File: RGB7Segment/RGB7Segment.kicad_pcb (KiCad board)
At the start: 2 copper layers, 34 x 31.5 mm, 14 parts, among them J1 Conn_01x04_Female, J2 Conn_01x04_Female

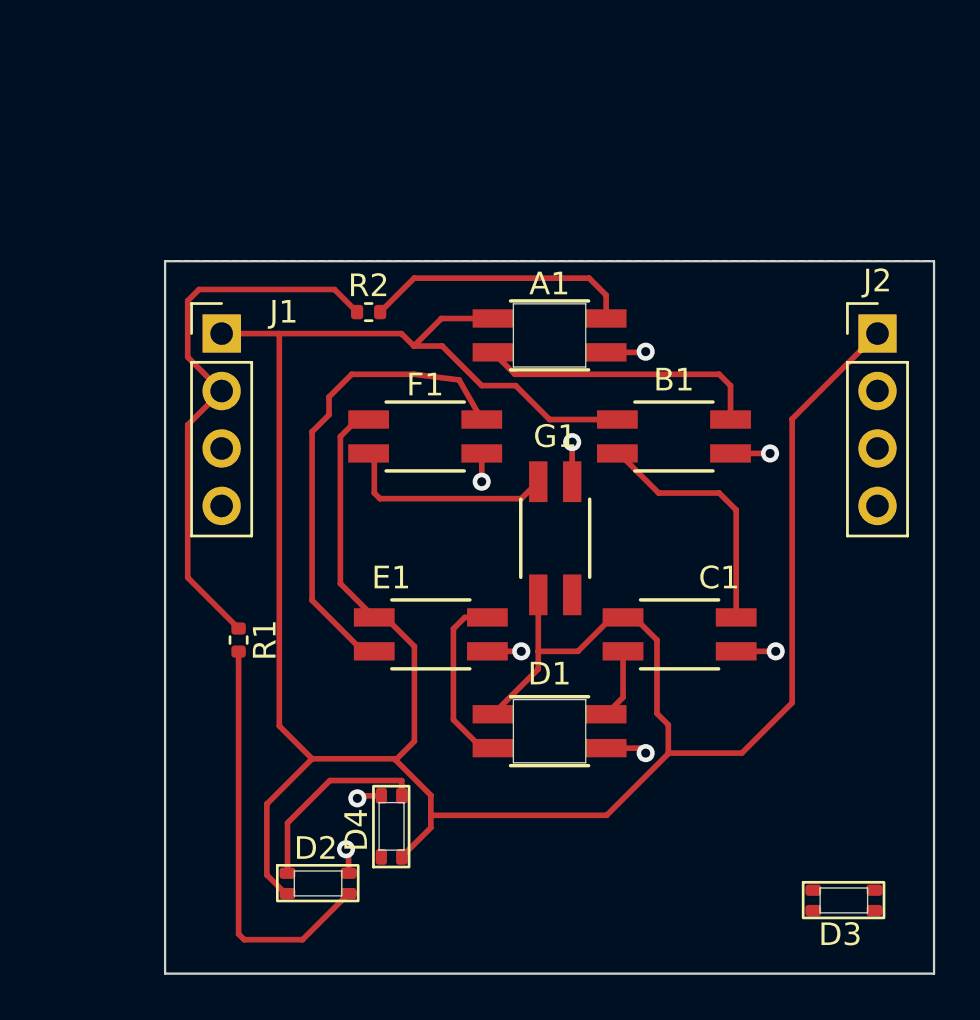
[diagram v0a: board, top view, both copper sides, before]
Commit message: Slotted/Cut Design Uploaded. Waiting on COnfirmation of Operation
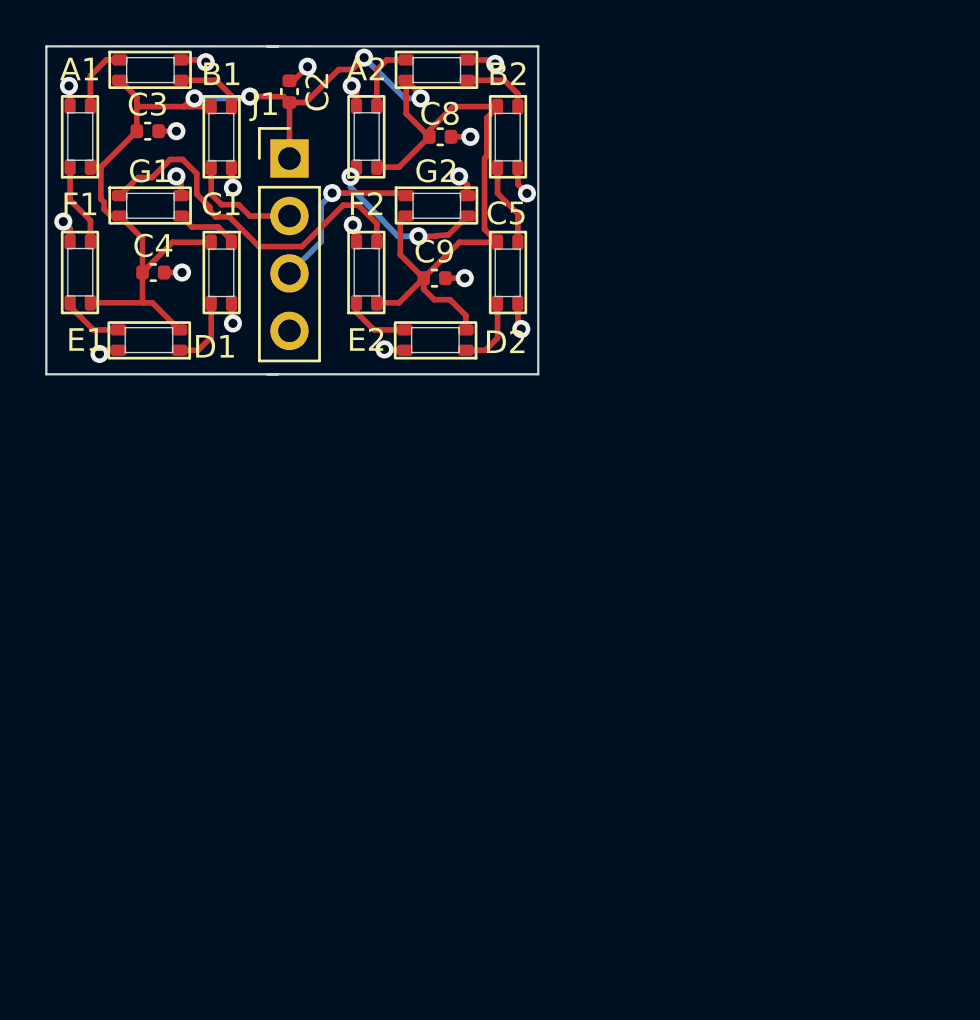
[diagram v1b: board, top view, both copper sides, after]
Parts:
- removed D3, D4: SK6812-E, Library:12-23C
- removed J2: Conn_01x04_Female, Connector_PinHeader_2.54mm:PinHeader_1x04_P2.54mm_Vertical
- removed R1, R2: 0, Resistor_SMD:R_0402_1005Metric
- added A2: SK6812-E, Library:12-23C, F.Cu at (192.7, 76.5)
- added B2: SK6812-E, Library:12-23C, F.Cu at (196.7, 77.7)
- added C2: 0.470u, Capacitor_SMD:C_0402_1005Metric, F.Cu at (187.5, 77.0)
- added C3: 0.1u, Capacitor_SMD:C_0402_1005Metric, F.Cu at (181.2, 78.8)
- added C4: 0.1u, Capacitor_SMD:C_0402_1005Metric, F.Cu at (181.5, 85.0)
- added C5: SK6812-E, Library:12-23C, F.Cu at (196.7, 83.7)
- added C8: 0.1u, Capacitor_SMD:C_0402_1005Metric, F.Cu at (194.2, 79.0)
- added C9: 0.1u, Capacitor_SMD:C_0402_1005Metric, F.Cu at (193.9, 85.2)
- added E2: SK6812-E, Library:12-23C, F.Cu at (191.4, 86.3)
- added F2: SK6812-E, Library:12-23C, F.Cu at (191.4, 80.3)
- added G2: SK6812-E, Library:12-23C, F.Cu at (192.7, 82.5)
- A1, D1: footprint Library:4960_ADA -> Library:12-23C
- B1: footprint Library:4960_Test2 -> Library:12-23C
- C1, G1: footprint Library:4960_Test4 -> Library:12-23C
- E1: footprint Library:4960_Test3 -> Library:12-23C
- F1: footprint Library:4960_Test1 -> Library:12-23C
- moved C1 27.0 mm to (184.0, 83.7), turned to -90 degrees
- moved D2 26.1 mm to (195.3, 87.5), turned to 180 degrees
- moved B1 25.1 mm to (184.0, 77.7), turned to -90 degrees
- moved D1 24.1 mm to (182.6, 87.5), turned to 180 degrees
- moved G1 24.0 mm to (180.0, 82.5), turned to 0 degrees
- moved A1 22.1 mm to (180.0, 76.5)
- moved E1 21.0 mm to (178.7, 86.3), turned to 90 degrees
- moved F1 19.0 mm to (178.7, 80.3), turned to 90 degrees
- moved J1 8.30 mm to (187.5, 80.0)
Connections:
- net +3V3 renamed VCC
- A1 pad 2: Net-(A1-Pad2) -> /F1
- A1 pad 4: Net-(R2-Pad2) -> /A1
- B1 pad 2: Net-(B1-Pad2) -> /A1
- B1 pad 4: Net-(A1-Pad2) -> /DIN
- C1 pad 2: /D1 -> /G1
- C1 pad 4: Net-(B1-Pad2) -> /C1
- D1 pad 2: Net-(D1-Pad2) -> /C1
- D2 pad 2: Net-(D2-Pad2) -> /C2
- D2 pad 4: Net-(D2-Pad4) -> /D2
- E1 pad 2: Net-(E1-Pad2) -> /D1
- E1 pad 4: Net-(D1-Pad2) -> /E1
- F1 pad 2: Net-(F1-Pad2) -> /E1
- F1 pad 4: Net-(E1-Pad2) -> /F1
- G1 pad 2: /D2 -> /E2
- G1 pad 4: Net-(F1-Pad2) -> /G1
- J1 pad 3: unconnected-(J1-Pad3) -> /DOUT
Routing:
- net VCC: track 130.3 -> 68.7 mm, vias 0 -> 4
- net Net-(E1-Pad2): track 21.2 -> 0.00 mm
- net /DIN: track 24.8 -> 5.04 mm
- net Net-(D2-Pad4): track 18.3 -> 0.00 mm
- net /E2: track 0.00 -> 16.1 mm
- net Net-(A1-Pad2): track 12.6 -> 0.00 mm
- net Net-(R2-Pad2): track 12.0 -> 0.00 mm
- net Net-(B1-Pad2): track 11.0 -> 0.00 mm
- net Net-(F1-Pad2): track 9.52 -> 0.00 mm
- net Net-(D2-Pad2): track 8.73 -> 0.00 mm
- net Net-(D1-Pad2): track 8.00 -> 0.00 mm
- net /DOUT: track 0.00 -> 7.65 mm, vias 0 -> 1
- net /G2: track 0.00 -> 7.44 mm, vias 0 -> 2
- net GND: track 13.8 -> 18.6 mm, vias 9 -> 19
- net /B2: track 0.00 -> 3.67 mm
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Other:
- board size 34 x 31.5 mm -> 21.8 x 14.5 mm
